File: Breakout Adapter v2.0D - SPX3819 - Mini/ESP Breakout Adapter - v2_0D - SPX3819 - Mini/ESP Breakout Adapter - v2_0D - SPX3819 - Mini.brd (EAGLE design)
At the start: 24.3 x 30.6 mm, 27 parts, among them U1 SPX3819

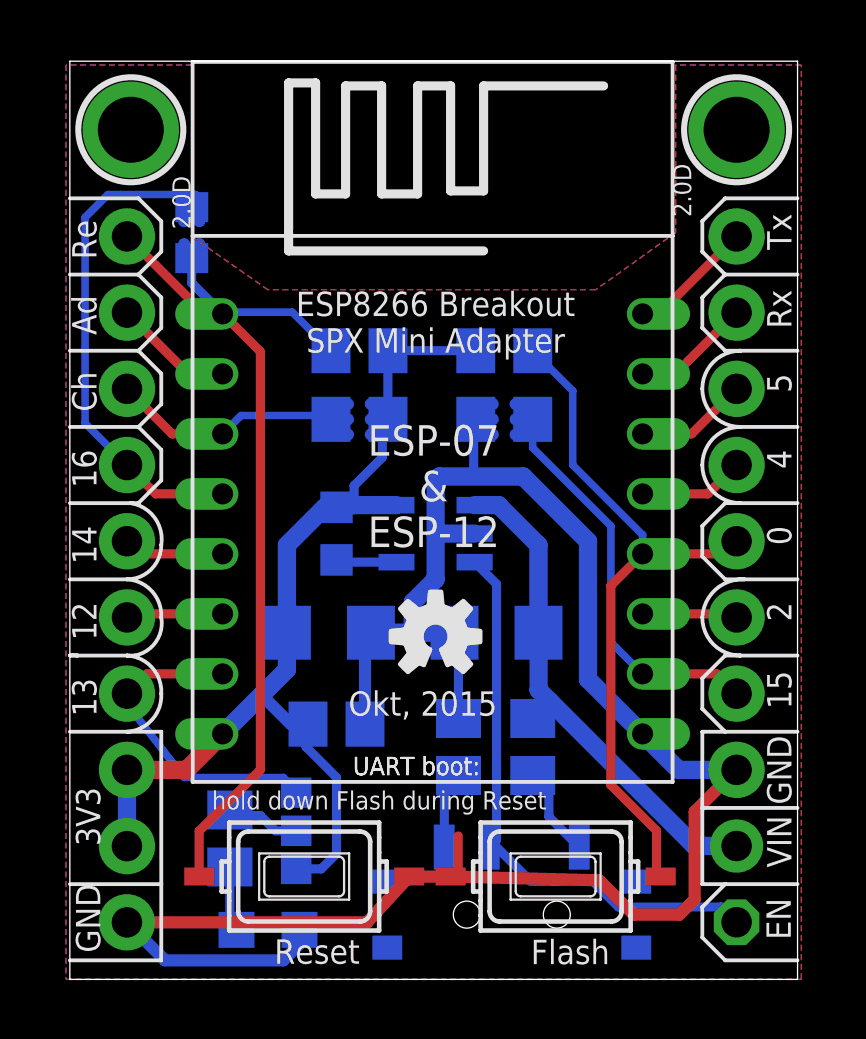
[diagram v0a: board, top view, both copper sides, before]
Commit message: mini änderung
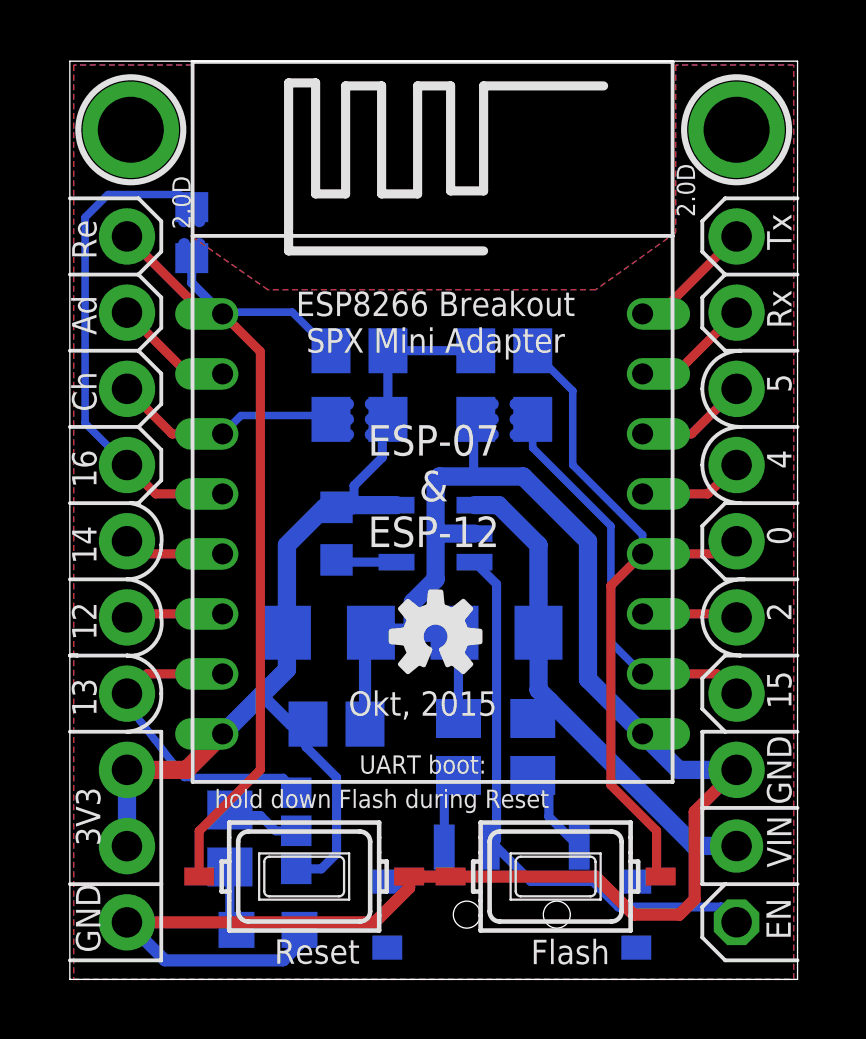
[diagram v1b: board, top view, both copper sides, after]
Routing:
- net GND: track 71.7 -> 70.7 mm
- net GPIO16: track 19.2 -> 18.6 mm
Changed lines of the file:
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@@
 <wire x1="22.606" y1="10.922" x2="21.336" y2="12.192" width="0.127" layer="21" curve="-90"/>
 <wire x1="21.336" y1="12.192" x2="22.733" y2="13.462" width="0.127" layer="21" curve="-90"/>
-<text x="4.9911" y="5.7912" size="0.6096" layer="21" ratio="12">hold down Flash during Reset</text>
-<text x="9.6901" y="6.9342" size="0.6096" layer="21" ratio="12">UART boot: </text>
-<text x="20.3581" y="27.3177" size="0.6096" layer="21" ratio="12" rot="R270">2.0D</text>
+<text x="5.08" y="5.842" size="0.6096" layer="21" ratio="12">hold down Flash during Reset</text>
+<text x="9.906" y="6.985" size="0.6096" layer="21" ratio="12">UART boot: </text>
+<text x="20.4851" y="27.3177" size="0.6096" layer="21" ratio="12" rot="R270">2.0D</text>
 <text x="12.446" y="23.0505" size="0.8128" layer="21" ratio="12" align="top-center">ESP8266 Breakout
 SPX Mini Adapter</text>
-<text x="9.6901" y="6.9342" size="0.6096" layer="21" ratio="12">UART boot: </text>
 <text x="4.2799" y="25.1333" size="0.6096" layer="21" ratio="12" rot="R90">2.0D</text>
 </plain>
@@
 <wire x1="5.346" y1="16.31" x2="3.121" y2="16.31" width="0.3048" layer="1"/>
 <wire x1="3.121" y1="16.31" x2="2.159" y2="17.272" width="0.3048" layer="1"/>
-<wire x1="4.445" y1="26.289" x2="1.524" y2="26.289" width="0.254" layer="16"/>
+<wire x1="3.898" y1="26.289" x2="1.524" y2="26.289" width="0.254" layer="16"/>
 <wire x1="1.524" y1="26.289" x2="0.762" y2="25.527" width="0.254" layer="16"/>
 <wire x1="0.762" y1="25.527" x2="0.762" y2="18.669" width="0.254" layer="16"/>
 <wire x1="0.762" y1="18.669" x2="2.159" y2="17.272" width="0.254" layer="16"/>
-<wire x1="4.445" y1="26.289" x2="4.445" y2="26.223" width="0.254" layer="16"/>
-<wire x1="4.445" y1="26.223" x2="4.318" y2="25.869" width="0.254" layer="16"/>
 <wire x1="4.064" y1="25.4" x2="4.064" y2="25.908" width="0.4064" layer="16"/>
-<wire x1="4.572" y1="25.4" x2="4.572" y2="26.162" width="0.4064" layer="16"/>
-<wire x1="4.064" y1="25.908" x2="4.511" y2="25.908" width="0.3048" layer="16"/>
-<wire x1="4.511" y1="25.908" x2="4.318" y2="25.869" width="0.3048" layer="16"/>
-<wire x1="4.572" y1="26.162" x2="4.318" y2="25.869" width="0.3048" layer="16"/>
+<wire x1="4.572" y1="25.4" x2="4.572" y2="26.123" width="0.4064" layer="16"/>
+<wire x1="4.279" y1="25.908" x2="4.511" y2="25.908" width="0.3048" layer="16"/>
+<wire x1="4.572" y1="26.162" x2="4.572" y2="26.123" width="0.4064" layer="16"/>
+<wire x1="4.572" y1="26.123" x2="4.318" y2="25.869" width="0.4064" layer="16"/>
+<wire x1="4.064" y1="25.908" x2="4.279" y2="25.908" width="0.3048" layer="16"/>
+<wire x1="4.279" y1="25.908" x2="4.318" y2="25.869" width="0.3048" layer="16"/>
+<wire x1="3.898" y1="26.289" x2="4.318" y2="25.869" width="0.254" layer="16"/>
 </signal>
 <signal name="GPIO14">
@@
 <wire x1="17.526" y1="10.13" x2="19.346" y2="8.31" width="0.6096" layer="16"/>
 <wire x1="13.782" y1="18.796" x2="13.716" y2="18.73" width="0.254" layer="16"/>
-<wire x1="2.157159375" y1="2.028784375" x2="10.164284375" y2="2.028784375" width="0.4064" layer="1"/>
-<wire x1="10.164284375" y1="2.028784375" x2="11.5645" y2="3.556" width="0.4064" layer="1"/>
+<wire x1="2.157159375" y1="2.028784375" x2="10.418284375" y2="2.028784375" width="0.4064" layer="1"/>
 <wire x1="11.5645" y1="3.556" x2="12.9465" y2="3.556" width="0.4064" layer="1"/>
 <wire x1="19.346" y1="8.31" x2="20.543359375" y2="7.112640625" width="0.6096" layer="16"/>
@@
 <wire x1="14.224" y1="18.796" x2="14.224" y2="18.288" width="0.3048" layer="16"/>
 <wire x1="13.782" y1="18.796" x2="14.224" y2="18.796" width="0.3048" layer="16"/>
-<wire x1="12.9465" y1="3.556" x2="17.907" y2="3.429" width="0.4064" layer="1"/>
-<wire x1="17.907" y1="3.429" x2="19.05" y2="2.286" width="0.4064" layer="1"/>
+<wire x1="17.78" y1="3.556" x2="19.05" y2="2.286" width="0.4064" layer="1"/>
 <wire x1="19.05" y1="2.286" x2="20.574" y2="2.286" width="0.4064" layer="1"/>
 <wire x1="20.574" y1="2.286" x2="21.082" y2="2.794" width="0.4064" layer="1"/>
@@
 <wire x1="7.366" y1="0.762" x2="3.42394375" y2="0.762" width="0.4064" layer="16"/>
 <wire x1="3.42394375" y1="0.762" x2="2.157159375" y2="2.028784375" width="0.4064" layer="16"/>
-<wire x1="13.2005" y1="3.6415" x2="13.2005" y2="4.9115" width="0.3048" layer="1"/>
 <wire x1="13.2005" y1="3.6415" x2="13.159" y2="3.6415" width="0.3048" layer="1"/>
-<wire x1="13.159" y1="3.6415" x2="12.9465" y2="3.556" width="0.3048" layer="1"/>
-<polygon width="0.3048" layer="1">
-<vertex x="0.127" y="0.127"/>
-<vertex x="24.638" y="0.127"/>
-<vertex x="24.638" y="30.607"/>
-<vertex x="20.447" y="30.607"/>
-<vertex x="20.447" y="25.019"/>
-<vertex x="17.78" y="23.114"/>
-<vertex x="6.858" y="23.114"/>
-<vertex x="4.318" y="24.892"/>
-<vertex x="4.318" y="30.607"/>
-<vertex x="0.127" y="30.607"/>
-</polygon>
 <contactref element="C2" pad="2"/>
 <wire x1="15.367" y1="16.891" x2="12.573" y2="16.891" width="0.6096" layer="16"/>
@@
 <wire x1="13.7461" y1="14.986" x2="12.446" y2="14.986" width="0.6096" layer="16"/>
 <polygon width="0.3048" layer="16">
-<vertex x="0.127" y="0.127"/>
-<vertex x="24.638" y="0.127"/>
-<vertex x="24.638" y="30.607"/>
+<vertex x="0.381" y="0.127"/>
+<vertex x="24.384" y="0.127"/>
+<vertex x="24.384" y="30.607"/>
 <vertex x="20.447" y="30.607"/>
 <vertex x="20.447" y="25.019"/>
@@
 <vertex x="4.318" y="24.892"/>
 <vertex x="4.318" y="30.607"/>
-<vertex x="0.127" y="30.607"/>
+<vertex x="0.381" y="30.607"/>
+</polygon>
+<wire x1="11.5645" y1="3.556" x2="11.5645" y2="3.175" width="0.4064" layer="1"/>
+<wire x1="11.5645" y1="3.175" x2="10.418284375" y2="2.028784375" width="0.4064" layer="1"/>
+<wire x1="13.159" y1="3.6415" x2="13.032" y2="3.6415" width="0.4064" layer="1"/>
+<wire x1="13.032" y1="3.6415" x2="12.9465" y2="3.556" width="0.4064" layer="1"/>
+<wire x1="12.9465" y1="3.556" x2="17.78" y2="3.556" width="0.4064" layer="1"/>
+<polygon width="0.3048" layer="1">
+<vertex x="0.381" y="0.127"/>
+<vertex x="24.384" y="0.127"/>
+<vertex x="24.384" y="30.607"/>
+<vertex x="20.447" y="30.607"/>
+<vertex x="20.447" y="25.019"/>
+<vertex x="17.78" y="23.114"/>
+<vertex x="6.858" y="23.114"/>
+<vertex x="4.318" y="24.892"/>
+<vertex x="4.318" y="30.607"/>
+<vertex x="0.381" y="30.607"/>
 </polygon>
 </signal>
@@
 <wire x1="4.5645" y1="3.556" x2="4.5645" y2="5.0725" width="0.3048" layer="1"/>
 <wire x1="4.5645" y1="5.0725" x2="6.604" y2="7.112" width="0.3048" layer="1"/>
-<wire x1="4.064" y1="24.638" x2="4.064" y2="24.384" width="0.4064" layer="16"/>
-<wire x1="4.572" y1="24.638" x2="4.318" y2="24.169" width="0.4064" layer="16"/>
-<wire x1="4.318" y1="24.169" x2="4.572" y2="24.384" width="0.4064" layer="16"/>
-<wire x1="4.572" y1="24.638" x2="4.064" y2="24.384" width="0.3048" layer="16"/>
+<wire x1="4.064" y1="24.638" x2="4.064" y2="24.13" width="0.4064" layer="16"/>
+<wire x1="4.318" y1="24.169" x2="4.318" y2="24.384" width="0.4064" layer="16"/>
+<wire x1="4.572" y1="24.638" x2="4.191" y2="24.257" width="0.3048" layer="16"/>
+<wire x1="4.191" y1="24.257" x2="4.064" y2="24.13" width="0.3048" layer="16"/>
+<wire x1="4.572" y1="24.638" x2="4.572" y2="24.13" width="0.4064" layer="16"/>
+<wire x1="4.318" y1="24.169" x2="4.279" y2="24.169" width="0.4064" layer="16"/>
+<wire x1="4.279" y1="24.169" x2="4.191" y2="24.257" width="0.4064" layer="16"/>
 </signal>
 <signal name="GPIO13">
